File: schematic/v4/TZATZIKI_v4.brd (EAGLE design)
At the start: 41 x 50 mm, 8 parts, among them J1 2X20-CHIP-HEADERS2X20CHIP_OFF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

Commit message: moved to eint3 for Card detection
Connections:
- net N$16: now also J1.AP-EINT3; no longer J1.CSID7
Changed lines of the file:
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@@
 <contactref element="SPI_TOP" pad="9"/>
 <contactref element="SDIO_TOP" pad="9"/>
-<contactref element="J1" pad="CSID7"/>
 <contactref element="SDIO_BOT" pad="9"/>
+<contactref element="J1" pad="AP-EINT3"/>
+<wire x1="28.5" y1="46.38" x2="47.117" y2="36.83" width="0" layer="19" extent="1-1"/>
 <wire x1="15.7" y1="48.68" x2="28.5" y2="46.38" width="0" layer="19" extent="1-16"/>
 <wire x1="29.2" y1="25.48" x2="28.5" y2="46.38" width="0" layer="19" extent="1-1"/>
 <wire x1="16.6" y1="25.08" x2="29.2" y2="25.48" width="0" layer="19" extent="1-16"/>
-<wire x1="46.863" y1="19.05" x2="29.2" y2="25.48" width="0" layer="19" extent="1-1"/>
 </signal>
 </signals>

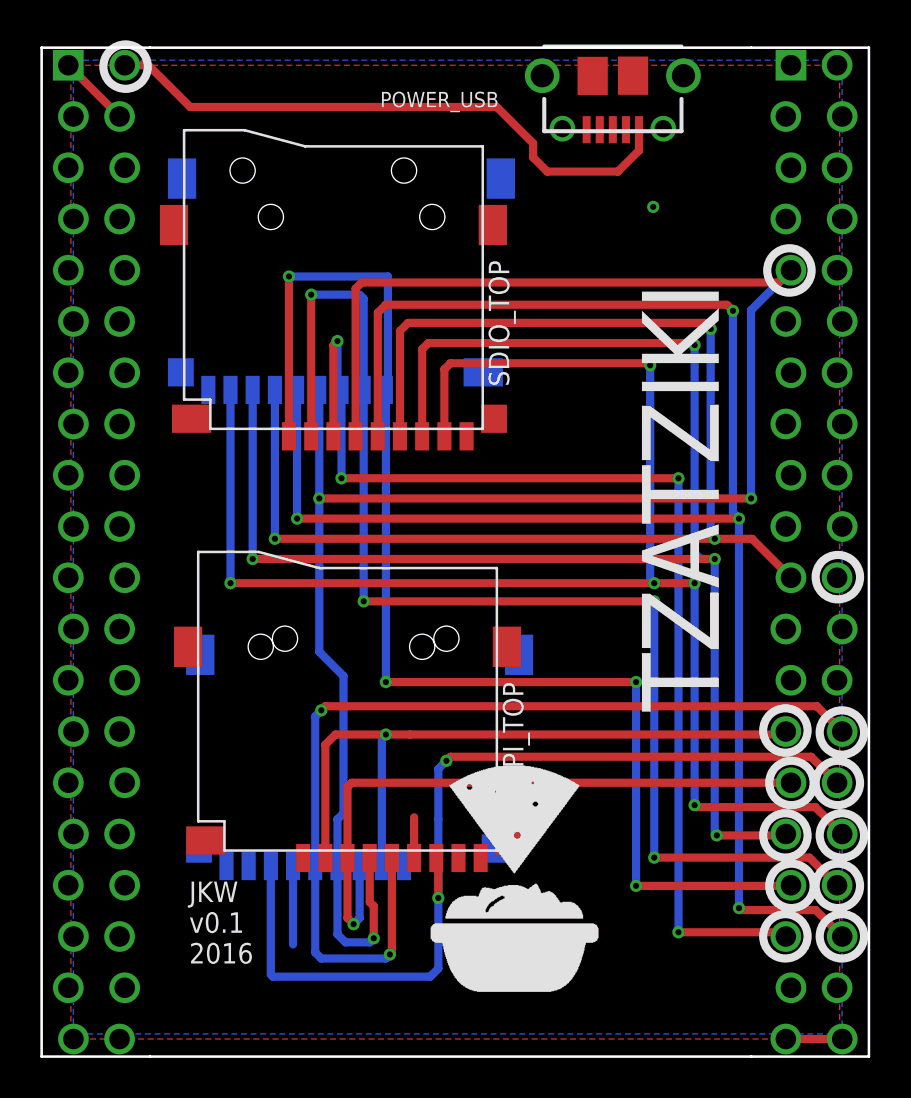
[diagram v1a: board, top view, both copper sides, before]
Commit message: added gerber
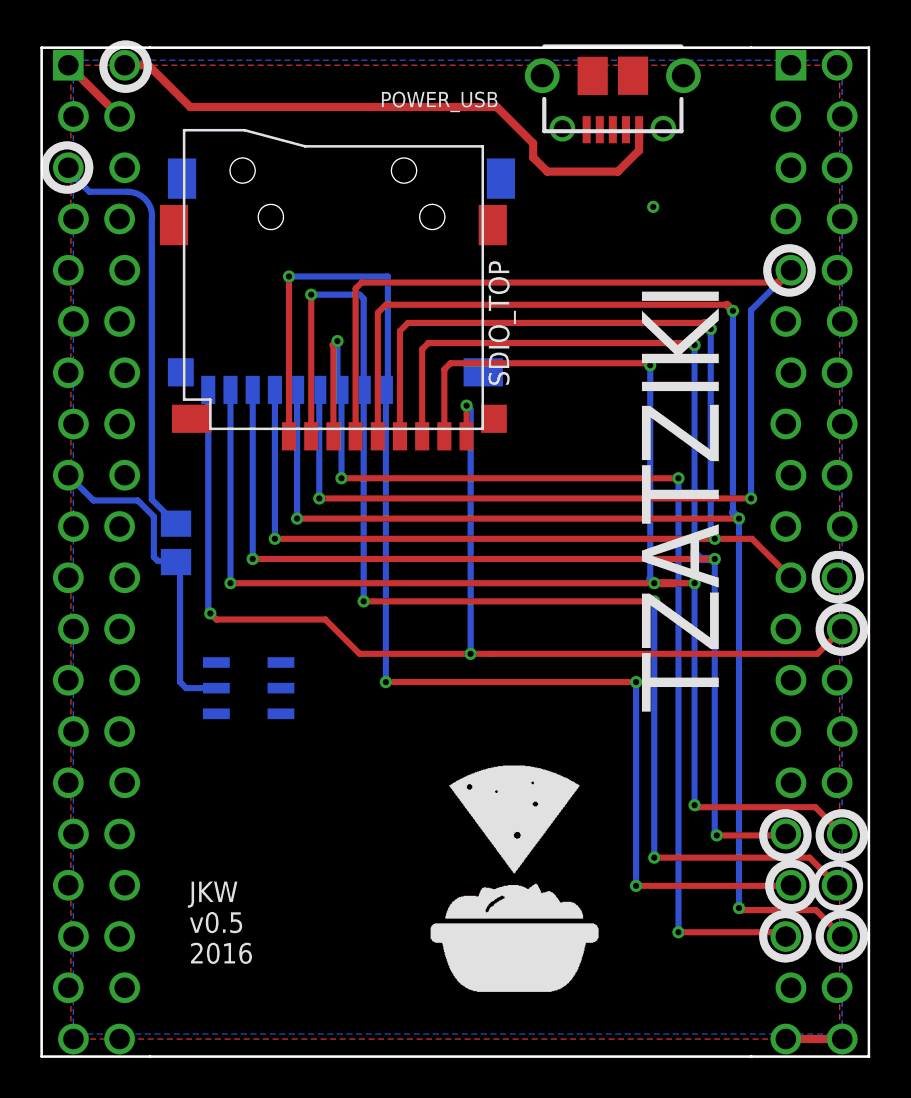
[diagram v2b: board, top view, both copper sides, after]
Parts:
- removed SPI_BOT, SPI_TOP: TF-HOLDER, JKW_CHIP:TF-PULL
- added R10: 2.2k, rcl:R0805
- added U2: DS2431P, JKW_CHIP:TSOC6
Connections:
- removed net N$11: J1.CSIPCK, SPI_BOT.2, SPI_TOP.2
- removed net N$12: J1.CSIHSYNC, SPI_BOT.3, SPI_TOP.3
- removed net N$13: J1.CSIVSYNC, SPI_BOT.7, SPI_TOP.7
- removed net N$14: J1.CSICK, SPI_BOT.5, SPI_TOP.5
- removed net VCC3V3: J1.VCC3V3
- new net LD2: J1.LCD-D2, R10.1, U2.2
- new net N$1: J1.VCC3V3, R10.2
- net GND: now also U2.1; no longer SPI_BOT.6, SPI_BOT.S1, SPI_BOT.S2, SPI_BOT.S3, SPI_BOT.S4, SPI_TOP.6, SPI_TOP.S1, SPI_TOP.S2, SPI_TOP.S3, SPI_TOP.S4
- net N$10: no longer SPI_BOT.4, SPI_TOP.4
- net N$16: no longer SPI_BOT.9, SPI_TOP.9
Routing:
- net N$16: track 0.00 -> 57.7 mm, vias 0 -> 3
- net N$14: track 47.3 -> 0.00 mm, vias 2 -> 0
- net N$13: track 46.4 -> 0.00 mm, vias 2 -> 0
- net N$11: track 35.3 -> 0.00 mm, vias 1 -> 0
- net N$12: track 32.0 -> 0.00 mm, vias 1 -> 0
- net N$10: track 96.7 -> 68.4 mm, vias 3 -> 2
- net N$1: track 0.00 -> 20.9 mm
- net LD2: track 0.00 -> 16.2 mm
- net GND: track 77.4 -> 71.5 mm
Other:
- board text added: "JKW v0.5 2016"
- board text removed: "JKW v0.1 2016"

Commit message: moved to correct subfolder
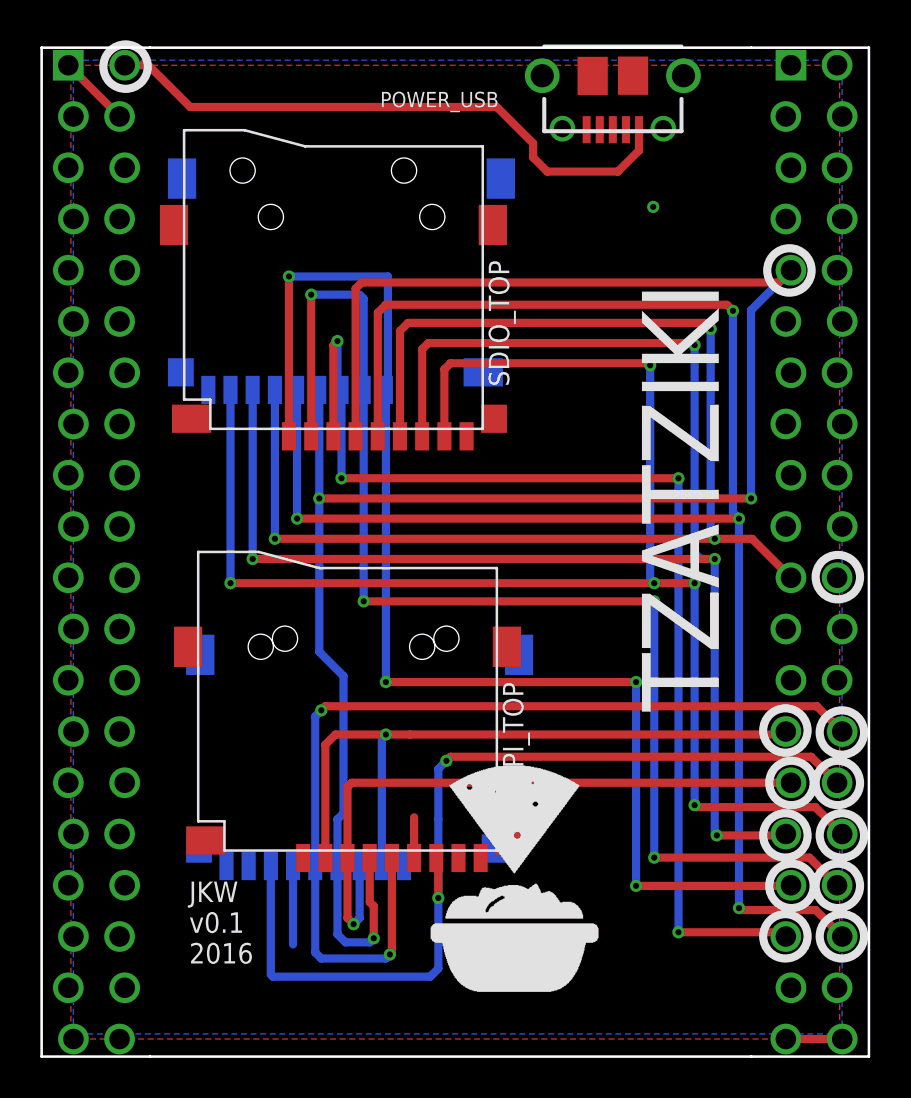
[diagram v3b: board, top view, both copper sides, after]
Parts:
- removed R10: 2.2k, rcl:R0805
- removed U2: DS2431P, JKW_CHIP:TSOC6
- added SPI_BOT, SPI_TOP: TF-HOLDER, JKW_CHIP:TF-PULL
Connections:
- removed net LD2: J1.LCD-D2, R10.1, U2.2
- removed net N$1: J1.VCC3V3, R10.2
- new net N$11: J1.CSIPCK, SPI_BOT.2, SPI_TOP.2
- new net N$12: J1.CSIHSYNC, SPI_BOT.3, SPI_TOP.3
- new net N$13: J1.CSIVSYNC, SPI_BOT.7, SPI_TOP.7
- new net N$14: J1.CSICK, SPI_BOT.5, SPI_TOP.5
- new net VCC3V3: J1.VCC3V3
- net GND: now also SPI_BOT.6, SPI_BOT.S1, SPI_BOT.S2, SPI_BOT.S3, SPI_BOT.S4, SPI_TOP.6, SPI_TOP.S1, SPI_TOP.S2, SPI_TOP.S3, SPI_TOP.S4; no longer U2.1
- net N$10: now also SPI_BOT.4, SPI_TOP.4
- net N$16: now also SPI_BOT.9, SPI_TOP.9
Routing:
- net N$16: track 57.7 -> 0.00 mm, vias 3 -> 0
- net N$14: track 0.00 -> 47.3 mm, vias 0 -> 2
- net N$13: track 0.00 -> 46.4 mm, vias 0 -> 2
- net N$11: track 0.00 -> 35.3 mm, vias 0 -> 1
- net N$12: track 0.00 -> 32.0 mm, vias 0 -> 1
- net N$10: track 68.4 -> 96.7 mm, vias 2 -> 3
- net N$1: track 20.9 -> 0.00 mm
- net LD2: track 16.2 -> 0.00 mm
- net GND: track 71.5 -> 77.4 mm
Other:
- board text added: "JKW v0.1 2016"
- board text removed: "JKW v0.5 2016"
